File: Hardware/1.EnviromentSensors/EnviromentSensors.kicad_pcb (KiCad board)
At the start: 2 copper layers, 70 x 70 mm, 14 parts, among them J2 Conn_01x05_Pin, U1 SHT4x, U2 BME680, U3 LPS22HB

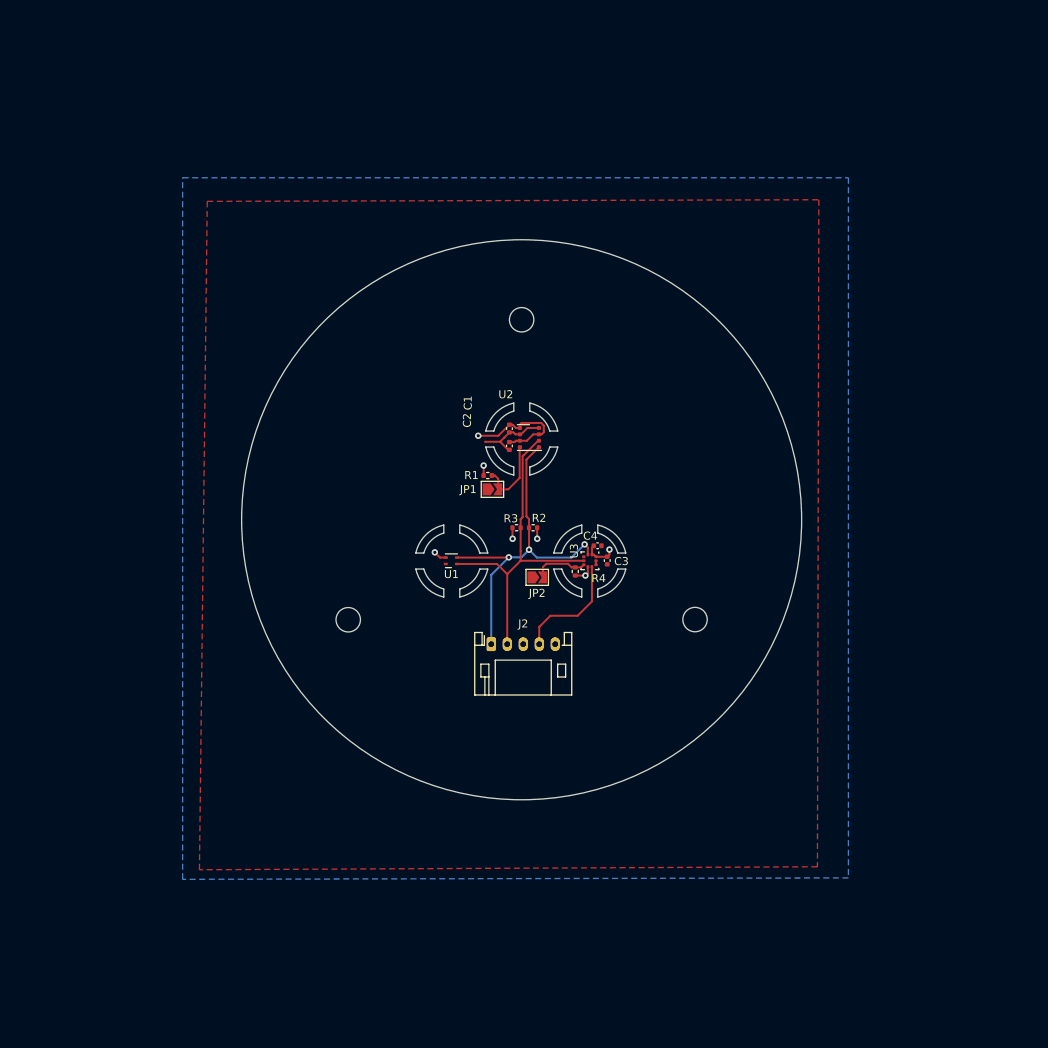
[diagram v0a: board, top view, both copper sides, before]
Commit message: Change PCB design
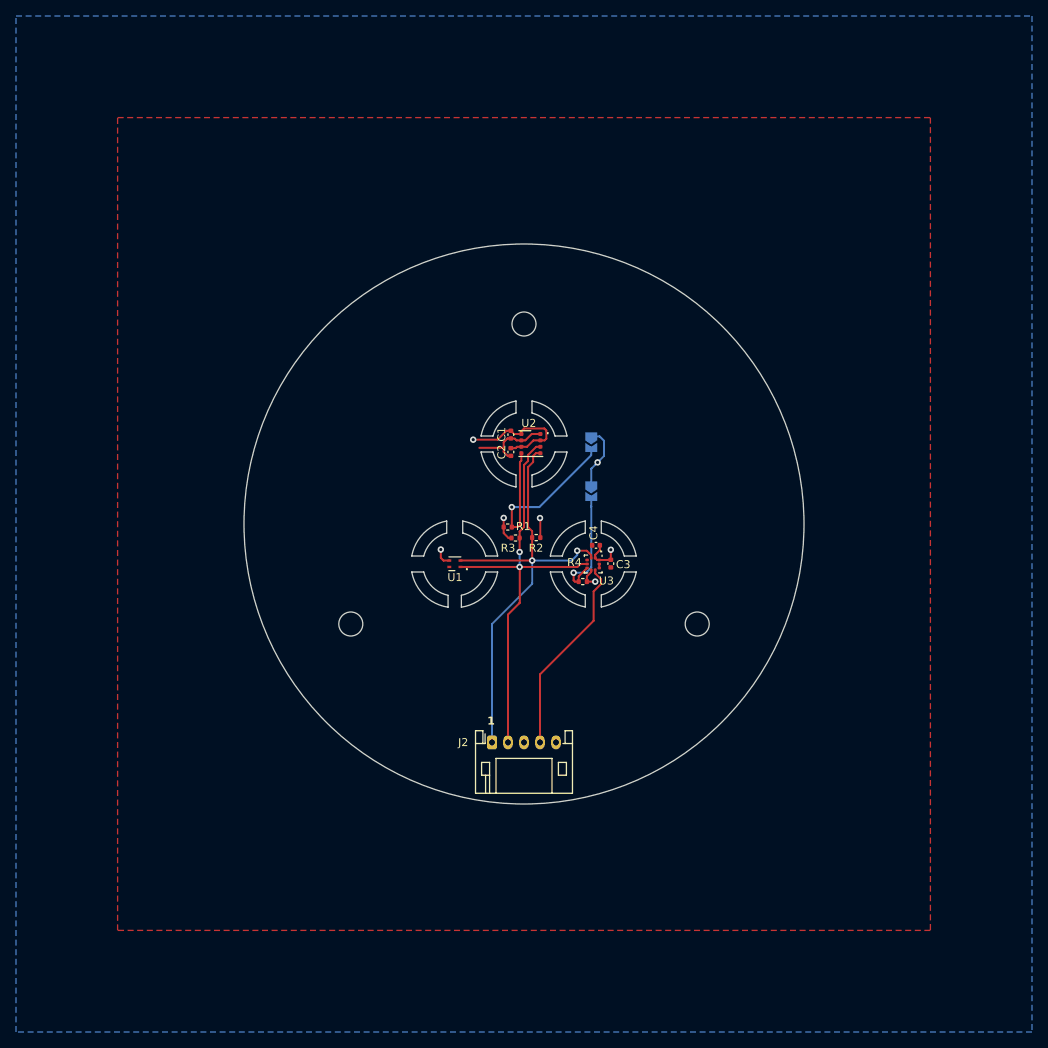
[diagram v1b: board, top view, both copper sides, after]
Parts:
- JP1, JP2: moved to B.Cu
- moved JP1 13.7 mm to (143.7, 75.3), turned to -90 degrees
- moved JP2 12.7 mm to (143.7, 81.4), turned to -90 degrees
- moved J2 12.3 mm to (131.3, 112.8)
- moved R1 6.90 mm to (133.3, 85.9)
- moved R4 1.58 mm to (142.6, 92.7), turned to 180 degrees
- moved R2 1.29 mm to (136.8, 87.2)
- moved R3 1.29 mm to (134.2, 87.3)
- moved C1 0.78 mm to (133.7, 74.4)
- moved U2 0.78 mm to (136.2, 75.5)
- moved C2 0.78 mm to (133.7, 76.5)
- moved C3 0.59 mm to (146.1, 90.5)
- moved U3 0.57 mm to (143.9, 90.5)
- moved U1 0.57 mm to (126.7, 90.5)
- moved C4 0.21 mm to (144.3, 88.2), turned to 180 degrees
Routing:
- net Net-(JP1-B): track 9.37 -> 26.2 mm, vias 0 -> 1
- net I2C_SDA: track 41.8 -> 54.9 mm, vias 0 -> 2
- net I2C_SCL: track 44.2 -> 57.2 mm, vias 3 -> 2
- net LPS22HB_INT: track 14.4 -> 25.0 mm
- net GND: track 9.77 -> 19.1 mm, vias 0 -> 1
- net Net-(JP2-B): track 6.88 -> 15.1 mm, vias 0 -> 1
- net +3.3V: track 27.6 -> 31.9 mm, vias 7 -> 6
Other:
- outline, holes or cut-outs redrawn
- board text added: "."
- board text added: "1"
- board text added: "BME680 Address: 0x76 - Closed 0x77 - Open"
- board text added: "LPS22HB Address: 0x5C - Closed 0x5D - Open"
